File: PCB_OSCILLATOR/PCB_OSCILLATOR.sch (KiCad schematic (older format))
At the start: 67 parts, among them J1 Jumper, J10 Jumper, J11 Jumper, J2 Jumper, J3 Jumper, J4 Jumper, J5 Jumper, J6 Jumper, J7 Jumper, J8 Jumper, J9 Jumper, P1 POWER SUPPLY, P2 SPI_AD5270_1, P3 SPI_AD5270_2, P4 SPI_AD9833_1, P5 SPI_AD9833_2, U1 AD5270, U2 AD8421, U3 AD9833, U4 AD5270, U5 AD8421, U6 AD9833, U7 ADG819

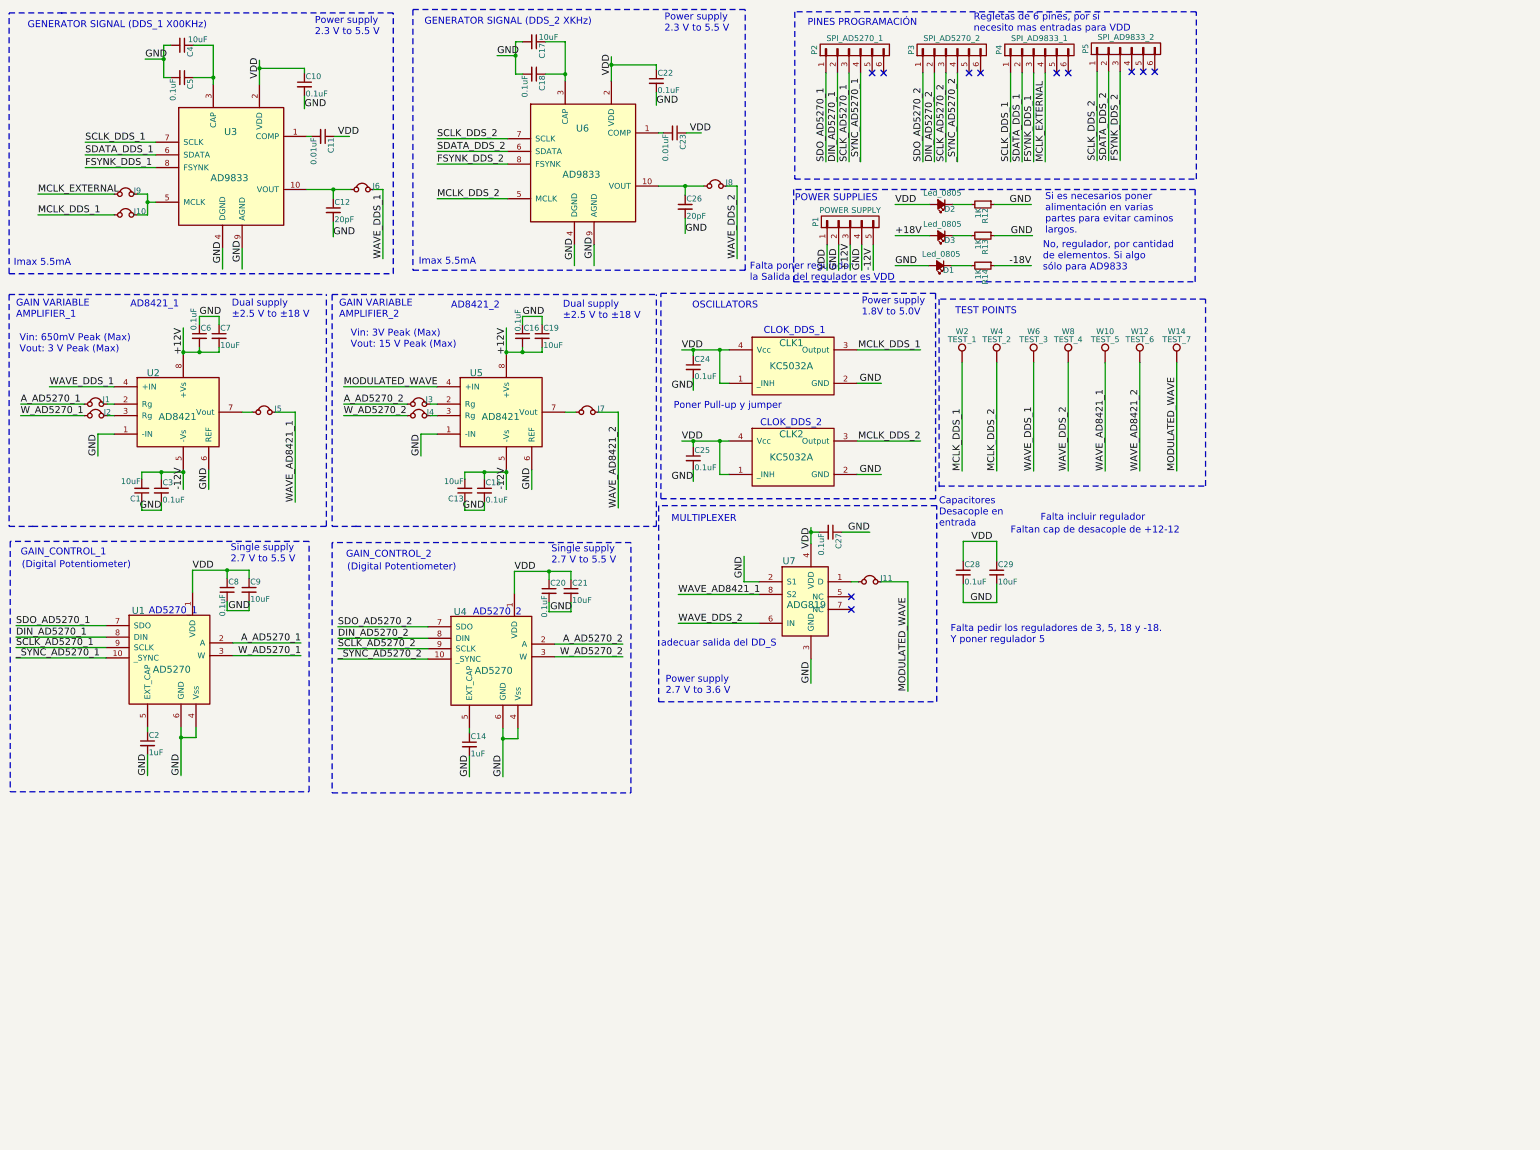
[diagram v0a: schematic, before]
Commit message: Algunos cambios Adicionales
//
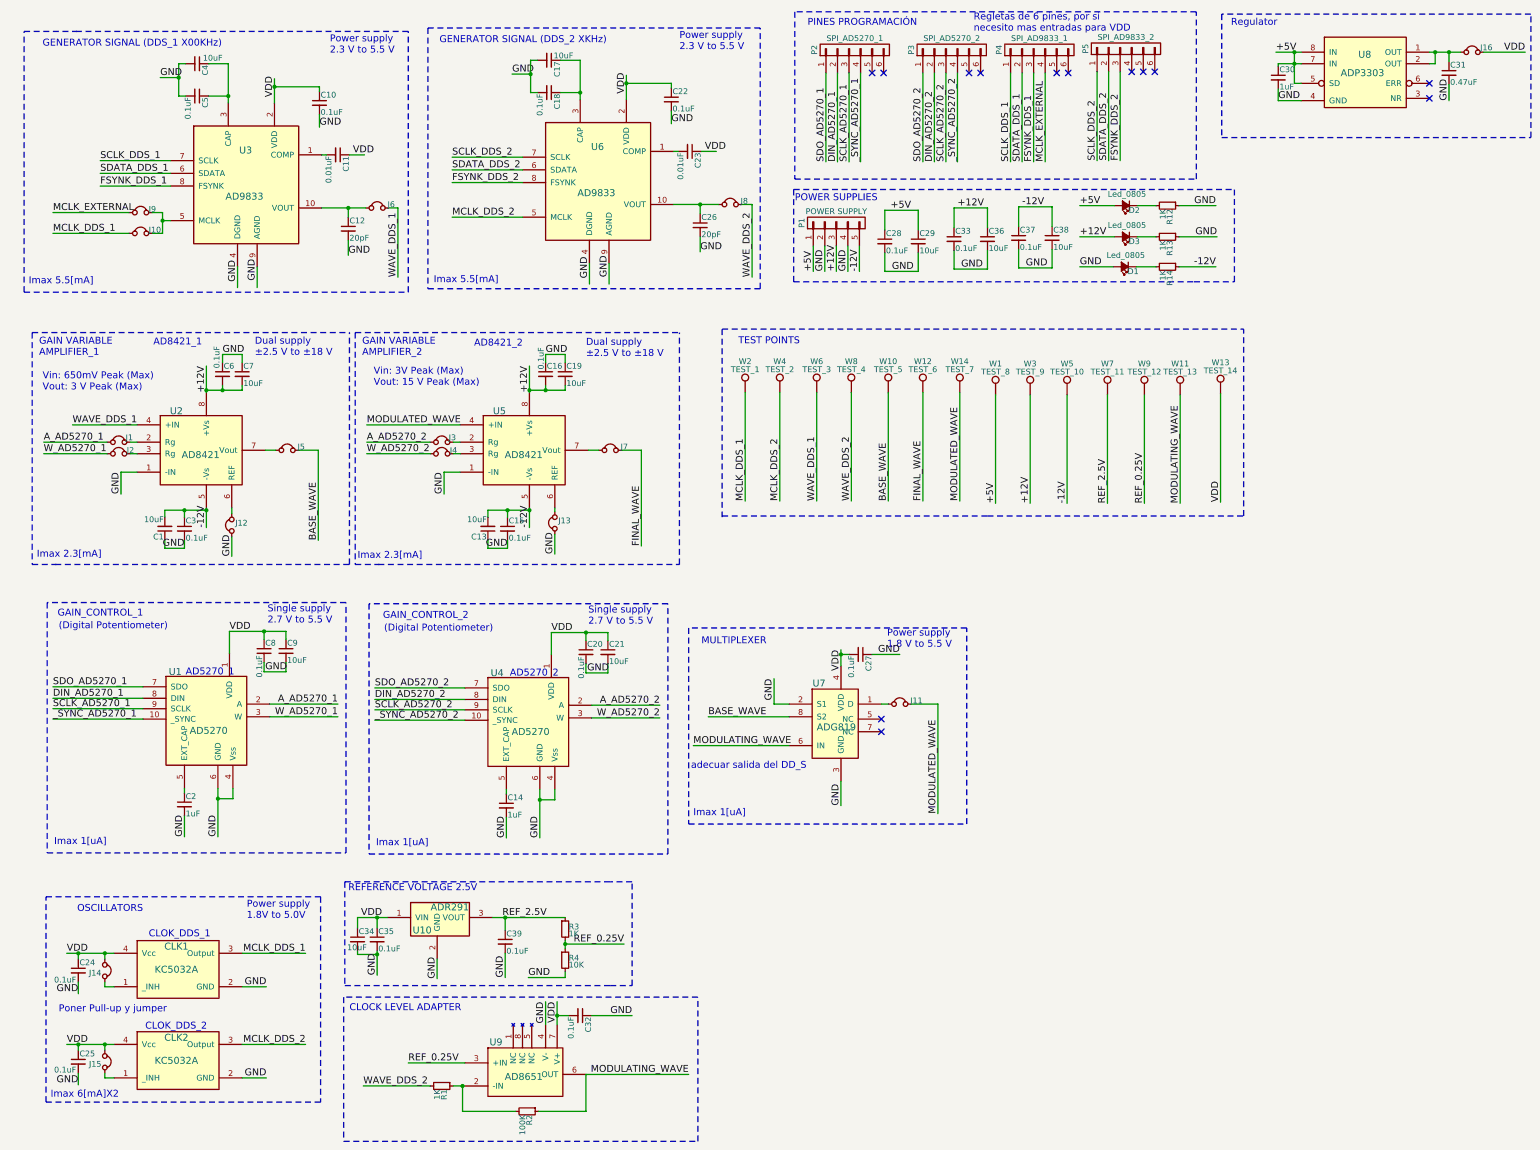
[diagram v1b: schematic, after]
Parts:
- added C30: 1uF, Capacitors_SMD:C_0805_HandSoldering, symbol 1uF
- added C31: 0.47uF, Capacitors_SMD:C_1206_HandSoldering, symbol 0.47uF
- added C32, C33, C35, C37, C39: 0.1uF, Resistors_SMD:R_0805_HandSoldering, symbol 0.1uF
- added C34, C36, C38: 10uF, Resistors_SMD:R_0805_HandSoldering, symbol 10uF
- added J12, J13, J14, J15, J16: Jumper, Pin_Headers:Pin_Header_Straight_1x02, symbol Jumper
- added R1, R3: 1K, Resistors_SMD:R_0805_HandSoldering, symbol 1K
- added R2: 100K, Resistors_SMD:R_0805_HandSoldering, symbol 100K
- added R4: 10K, Resistors_SMD:R_0805_HandSoldering, symbol 10K
- added U10: ADR291, TO_SOT_Packages_THT:TO-92_Inline_Narrow_Oval, symbol ADR291
- added U8: ADP3303, Housings_SOIC:SOIC-8_3.9x4.9mm_Pitch1.27mm, symbol ADP3303
- added U9: AD8651, Housings_SOIC:SOIC-8_3.9x4.9mm_Pitch1.27mm, symbol AD8651
- added W1: TEST_8, Measurement_Points:Measurement_Point_Round-TH_Small, symbol TEST_1P
- added W11: TEST_13, Measurement_Points:Measurement_Point_Round-TH_Small, symbol TEST_1P
- added W13: TEST_14, Measurement_Points:Measurement_Point_Round-TH_Small, symbol TEST_1P
- added W3: TEST_9, Measurement_Points:Measurement_Point_Round-TH_Small, symbol TEST_1P
- added W5: TEST_10, Measurement_Points:Measurement_Point_Round-TH_Small, symbol TEST_1P
- added W7: TEST_11, Measurement_Points:Measurement_Point_Round-TH_Small, symbol TEST_1P
- added W9: TEST_12, Measurement_Points:Measurement_Point_Round-TH_Small, symbol TEST_1P
- C1, C13, C19, C7: footprint Resistors_SMD:R_0805_HandSoldering -> Capacitors_SMD:C_1206_HandSoldering; 25V 490-5523-2-ND -> (none); CAP TANT 10UF 16V 10% 1206 (none) -> 478-8235-2-ND
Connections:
- net labels added: +5V, BASE_WAVE, FINAL_WAVE, MODULATING_WAVE, REF_0.25V, REF_2.5V
- net labels removed: +18V, -18V, WAVE_AD8421_1, WAVE_AD8421_2
- wire segments 206 -> 268
- no-connect marks 11 -> 13
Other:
- note added: "CLOCK LEVEL ADAPTER"
- note added: "Imax 1[uA]"
- note added: "Imax 2.3[mA]"
- note added: "Imax 5.5[mA]"
- note added: "Imax 6[mA]X2"
- note added: "Power supply\n1.8 V to 5.5 V"
- note added: "REFERENCE VOLTAGE 2.5V"
- note added: "Regulator"
- note removed: "Capacitores\nDesacople en\nentrada\n"
- note removed: "Falta incluir regulador"
- note removed: "Falta pedir los reguladores de 3, 5, 18 y -18.\nY poner regulador 5"
- note removed: "Falta poner regulador\nla Salida del regulador es VDD"
- note removed: "Faltan cap de desacople de +12-12"
- note removed: "Imax 5.5mA"
- note removed: "No, regulador, por cantidad \nde elementos. Si algo \nsólo para AD9833"
- note removed: "Power supply\n2.7 V to 3.6 V"
- note removed: "Si es necesarios poner \nalimentación en varias \npartes para evitar caminos\nlargos."
- moved on the sheet: C1, C10, C11, C12, C13, C14, C15, C16, C17, C18, C19, C2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
